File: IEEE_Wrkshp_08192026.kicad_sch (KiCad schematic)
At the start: 21 parts, among them J1 Screw_Terminal_01x03, J2 Screw_Terminal_01x03, Q1 2SD600, U1 TLV172IDCK

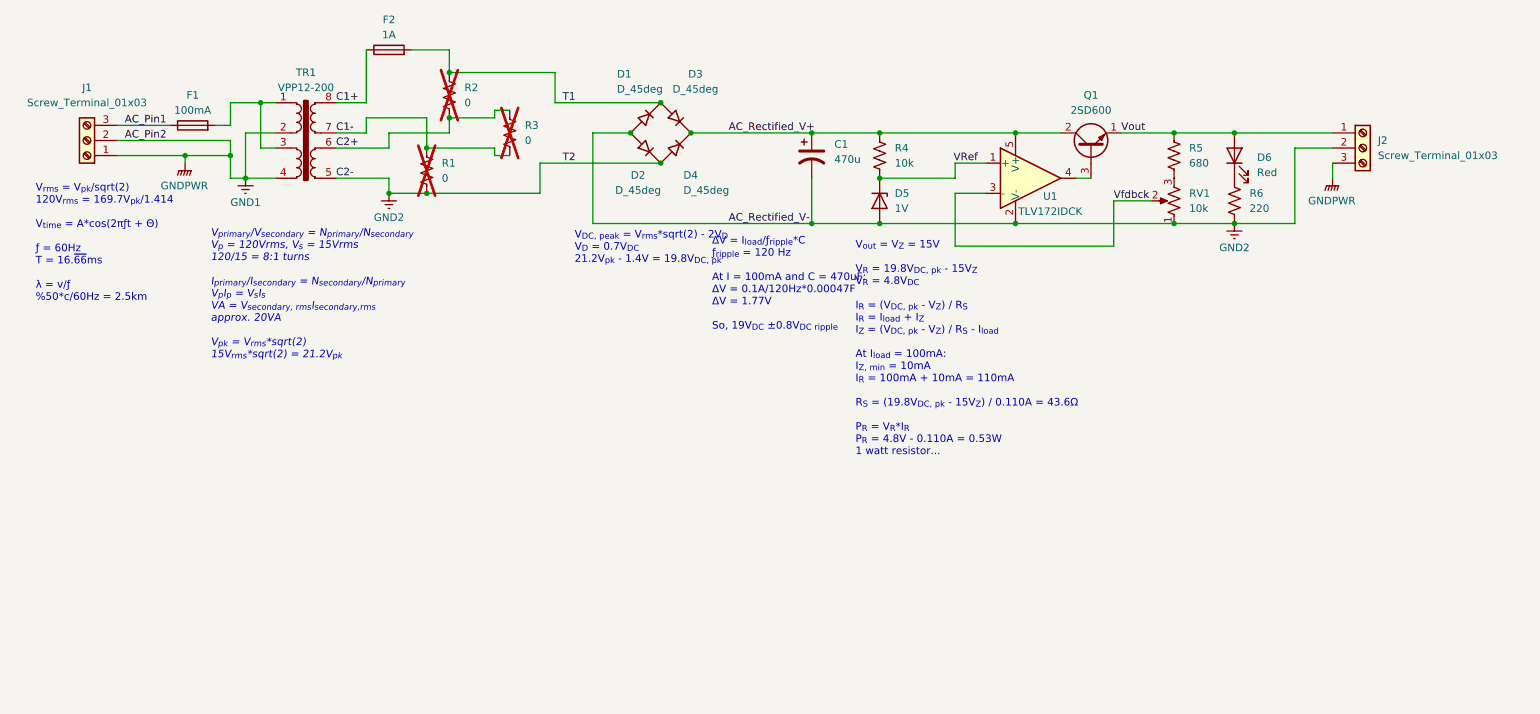
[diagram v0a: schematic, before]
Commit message: Almost Done
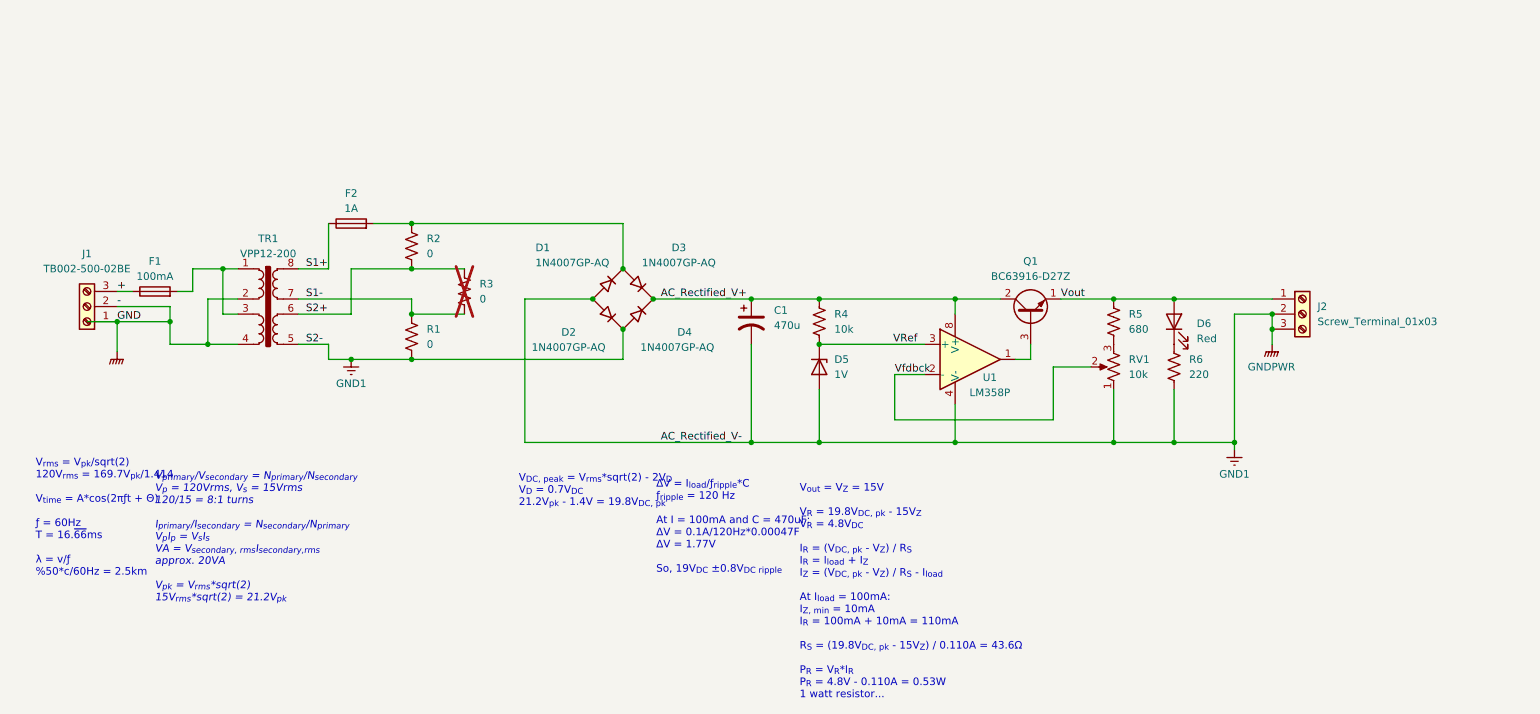
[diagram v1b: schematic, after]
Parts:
- D1, D2, D3, D4: value D_45deg -> 1N4007GP-AQ
- J1: value Screw_Terminal_01x03 -> TB002-500-02BE
- Q1: value 2SD600 -> BC63916-D27Z
- R1, R2: now fitted
- U1: value TLV172IDCK -> LM358P
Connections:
- net AC_Rectified_V+: now also U1.8 (V+); no longer U1.5 (V+)
- net GND1: now also C1.2, D1.2 (A), D2.1 (K), D2.2 (A), D4.2 (A), D5.2 (A), J2.2 (Pin_2), R1.2, R6.2, RV1.1, TR1.5, U1.4 (V-)
- net VRef: now also U1.3 (+); no longer U1.1 (+)
- net Vfdbck: now also U1.2 (-); no longer U1.3 (-)
- net at Q1.3 (B): now also U1.1; no longer U1.4
- net AC_Pin1 renamed +
- net C1+ renamed S1+
- net C1- renamed S1-
- net C2+ renamed S2+
- removed net GND2: C1.2, D1.2 (A), D2.1 (K), D2.2 (A), D4.2 (A), D5.2 (A), J2.2 (Pin_2), R1.2, R6.2, RV1.1, TR1.5, U1.2 (V-)
- net T1: no longer names the net of D1.1 (K), D3.2 (A), F2.2, R2.1
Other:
- company: Lamar University | IEEE -> Lamar University
- title: IEEE Workshop PCB | Electronics | Hardware | Design Engineering -> IEEE PCB Design Series 2026
- moved on the sheet: C1, D1, D2, D3, D4, D5, D6, F1, F2, J1, J2, Q1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
